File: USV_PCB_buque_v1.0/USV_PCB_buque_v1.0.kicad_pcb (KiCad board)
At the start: 2 copper layers, 6 parts, among them U1 Radio, U2 BluePill

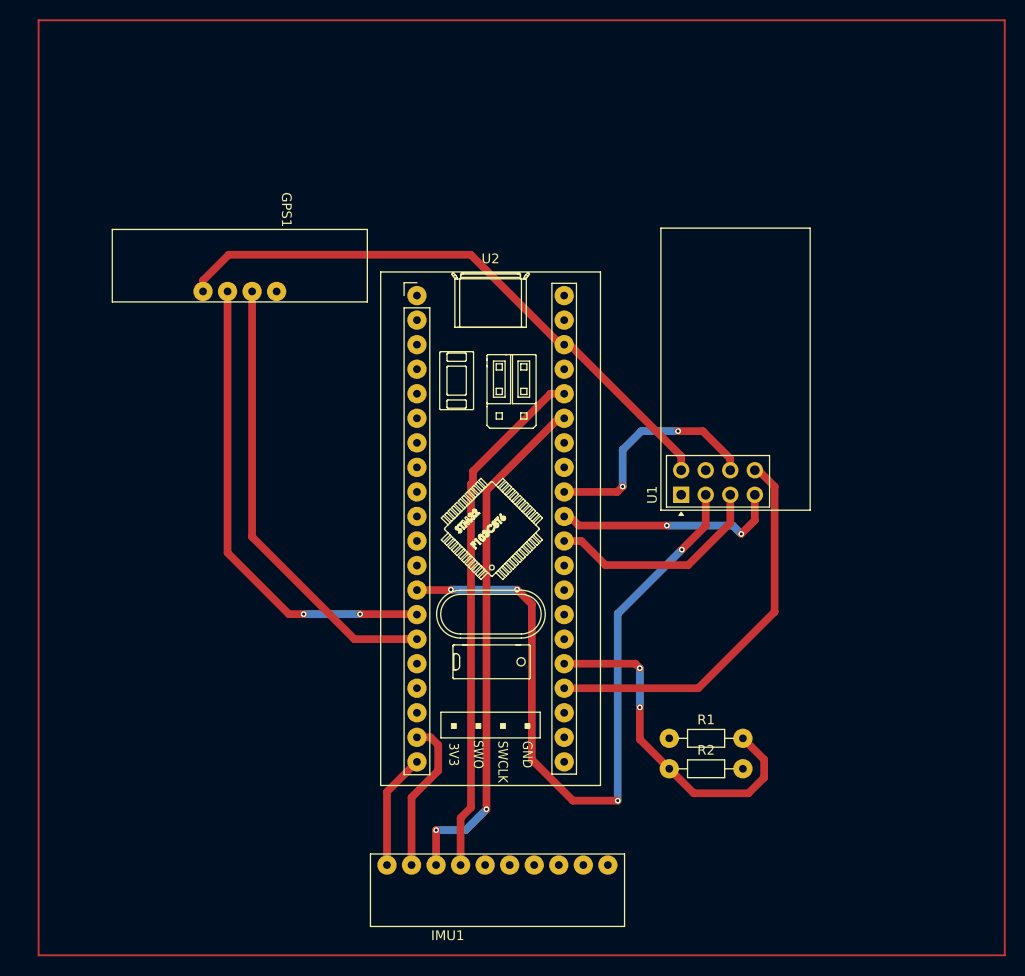
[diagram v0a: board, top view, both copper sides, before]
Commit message: Cambios hechos la noche de entrega
escuchando virus
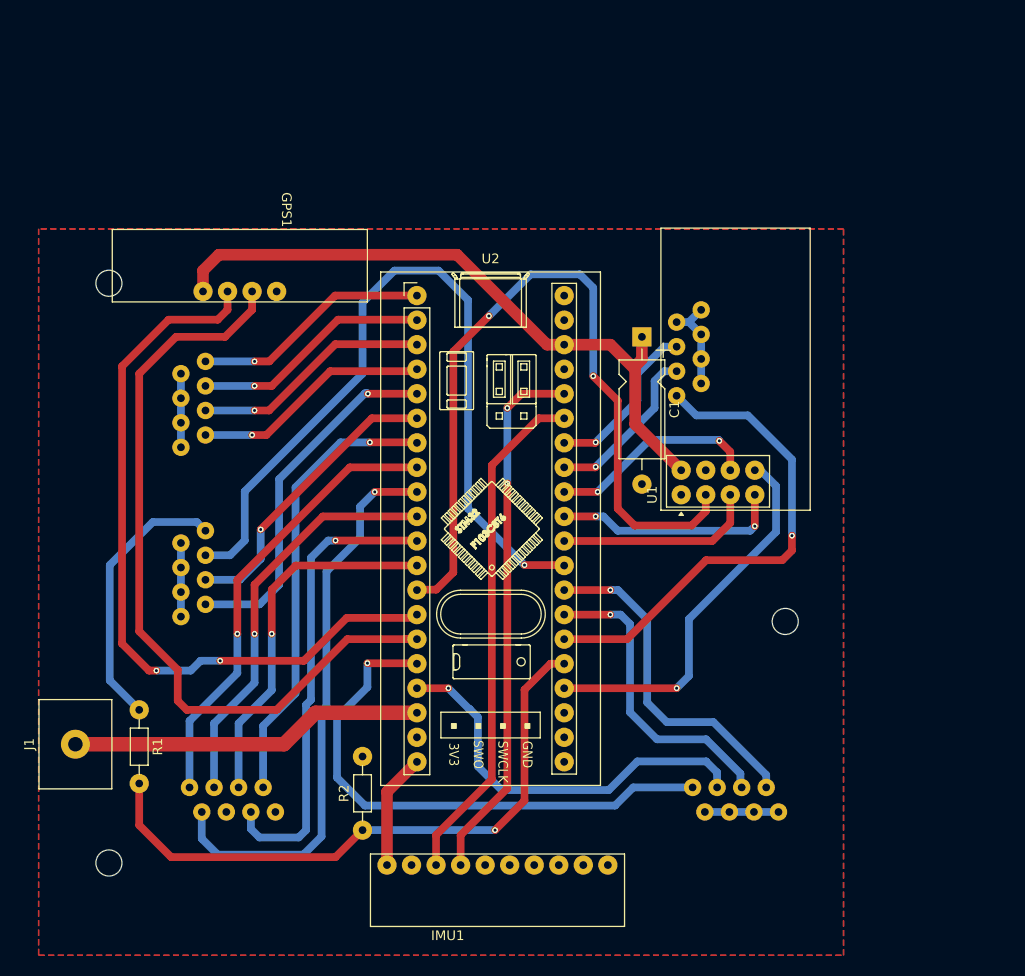
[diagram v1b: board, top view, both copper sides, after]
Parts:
- added C1: 10uF, Capacitor_THT:CP_Axial_L10.0mm_D4.5mm_P15.00mm_Horizontal, F.Cu at (235.2, 50.5)
- added J1: Bornera alimentación, TerminalBlock_MetzConnect:TerminalBlock_MetzConnect_360271_1x01_Horizontal_ScrewM3.0_Boxed, F.Cu at (176.5, 92.7)
- added LAN1: ~, USV_componentes:LAN, B.Cu at (168.4, 57.5)
- added LAN2: ~, USV_componentes:LAN, B.Cu at (192.8, 118.8)
- added LAN3: ~, USV_componentes:LAN, B.Cu at (260.4, 52.2)
- added LAN4: ~, USV_componentes:LAN, B.Cu at (244.9, 118.8)
- added LAN5: ~, USV_componentes:LAN, B.Cu at (168.4, 75.1)
- added REF**: Agujero de Montaje, MountingHole:MountingHole_2.7mm, F.Cu at (180.0, 105.0)
- added REF**: Agujero de Montaje, MountingHole:MountingHole_2.7mm, F.Cu at (250.0, 80.0)
- added REF**: Agujero de Montaje, MountingHole:MountingHole_2.7mm, F.Cu at (180.0, 45.0)
- moved R1 54.9 mm to (183.1, 89.2), turned to -90 degrees
- moved R2 32.4 mm to (206.2, 101.6), turned to 90 degrees
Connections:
- net Net-(U2-PA0) renamed /Vbat_test
- U2 pad 29: Ib sensor -> Net-(LAN5-Green)
- U2 pad 5: M1 signal -> Net-(LAN5-Orange)
- U2 pad 6: M2 signal -> Net-(LAN5-Blue)
- U2 pad 7: servo timón -> Net-(LAN2-Orange)
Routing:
- net Net-(LAN5-Green): track 0.00 -> 81.9 mm, vias 0 -> 1
- net Net-(LAN2-Brown-w): track 0.00 -> 58.9 mm, vias 0 -> 1
- net Net-(LAN4-Brown): track 0.00 -> 57.1 mm, vias 0 -> 1
- net Net-(LAN3-Brown): track 0.00 -> 51.5 mm, vias 0 -> 1
- net Net-(LAN2-Green-w): track 0.00 -> 48.3 mm, vias 0 -> 1
- net Net-(LAN2-Orange): track 0.00 -> 47.0 mm, vias 0 -> 1
- net Net-(LAN2-Brown): track 0.00 -> 46.9 mm, vias 0 -> 1
- net Net-(LAN2-Green): track 0.00 -> 42.5 mm, vias 0 -> 1
- net Net-(LAN4-Green): track 0.00 -> 41.7 mm, vias 0 -> 1
- net Net-(LAN2-Blue): track 0.00 -> 38.0 mm, vias 0 -> 1
- net Net-(LAN5-Orange): track 0.00 -> 37.4 mm, vias 0 -> 1
- net +5V: track 0.00 -> 36.7 mm
- net Net-(LAN4-Orange): track 0.00 -> 35.2 mm, vias 0 -> 1
- net Net-(GPS1-TX): track 48.1 -> 81.2 mm
- net Net-(LAN4-Blue): track 0.00 -> 31.9 mm, vias 0 -> 1
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- added copper zone on B.Cu, net GND
- added copper zone on F.Cu, net GND
